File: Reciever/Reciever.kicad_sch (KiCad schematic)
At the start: 3 parts, among them J2 USB_A, U1 ESP32-S3-MINI-1, U2 MCP1700x-330xxTT

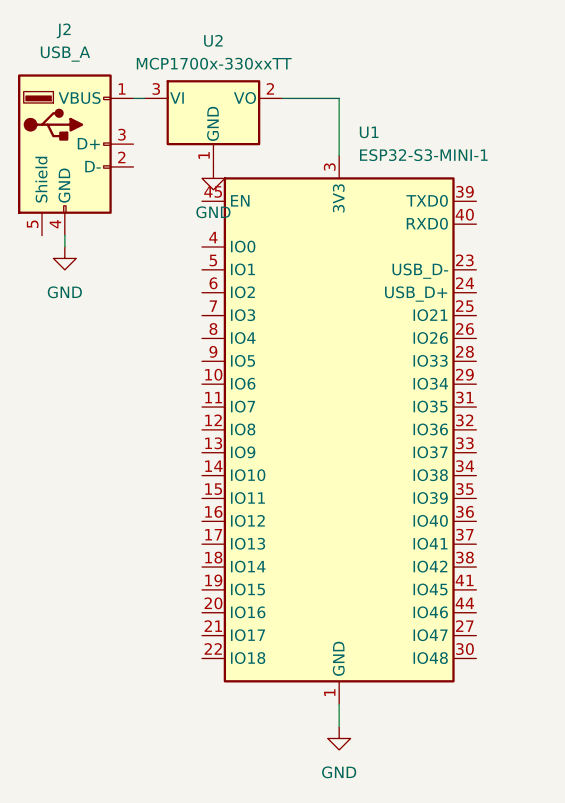
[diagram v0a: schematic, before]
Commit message: UPDATING RECIEVER
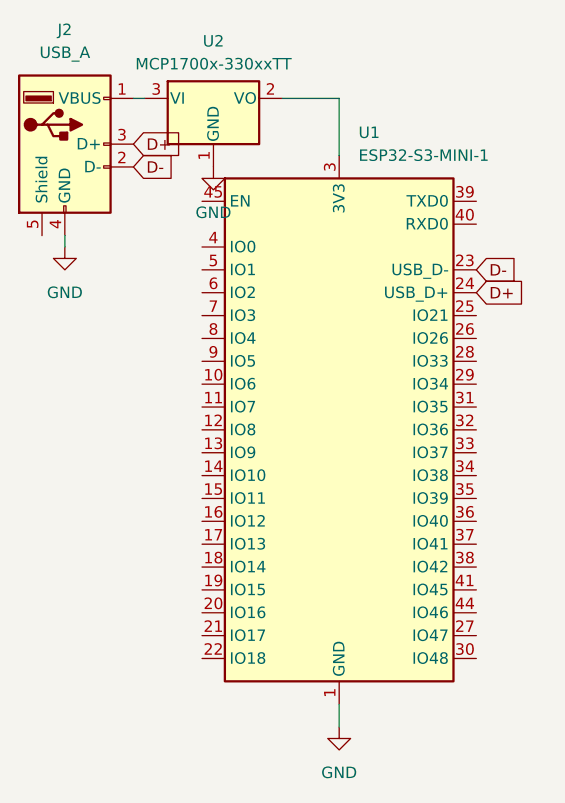
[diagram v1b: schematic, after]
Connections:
- net D-: now reaches U1.23 (USB_D-)
- net D-: now also J2.2 (D-)
- net D+: now reaches U1.24 (USB_D+)
- net D+: now also J2.3 (D+)
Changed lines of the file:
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@@
+		)
+	)
+	(global_label "D-"
+		(shape input)
+		(at 58.42 33.02 0)
+		(fields_autoplaced yes)
+		(effects
+			(font
+				(size 1.27 1.27)
+			)
+			(justify left)
+		)
+		(property "Intersheetrefs" "${INTERSHEET_REFS}"
+			(at 64.2476 33.02 0)
+			(effects
+				(font
+					(size 1.27 1.27)
+				)
+				(justify left)
+				(hide yes)
+			)
+		)
+	)
+	(global_label "D+"
+		(shape input)
+		(at 58.42 30.48 0)
+		(fields_autoplaced yes)
+		(effects
+			(font
+				(size 1.27 1.27)
+			)
+			(justify left)
+		)
+		(property "Intersheetrefs" "${INTERSHEET_REFS}"
+			(at 64.2476 30.48 0)
+			(effects
+				(font
+					(size 1.27 1.27)
+				)
+				(justify left)
+				(hide yes)
+			)
+		)
+	)
+	(global_label "D-"
+		(shape input)
+		(at 96.52 44.45 0)
+		(fields_autoplaced yes)
+		(effects
+			(font
+				(size 1.27 1.27)
+			)
+			(justify left)
+		)
+		(property "Intersheetrefs" "${INTERSHEET_REFS}"
+			(at 102.3476 44.45 0)
+			(effects
+				(font
+					(size 1.27 1.27)
+				)
+				(justify left)
+				(hide yes)
+			)
+		)
+	)
+	(global_label "D+"
+		(shape input)
+		(at 96.52 46.99 0)
+		(fields_autoplaced yes)
+		(effects
+			(font
+				(size 1.27 1.27)
+			)
+			(justify left)
+		)
+		(property "Intersheetrefs" "${INTERSHEET_REFS}"
+			(at 102.3476 46.99 0)
+			(effects
+				(font
+					(size 1.27 1.27)
+				)
+				(justify left)
+				(hide yes)
+			)
 		)
 	)
